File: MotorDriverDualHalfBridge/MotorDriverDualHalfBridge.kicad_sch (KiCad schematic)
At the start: 42 parts, among them J3 Batt+, J3 Batt-, J3 Motor Bottom Connection, J3 Motor Middle Connection, J3 Motor Upper Connection, J6 Conn_01x04, Q1 IAUA250N04S6N005, Q2 IAUA250N04S6N005, U1 2ED21824S06J, U2 EL817, U3 EL817

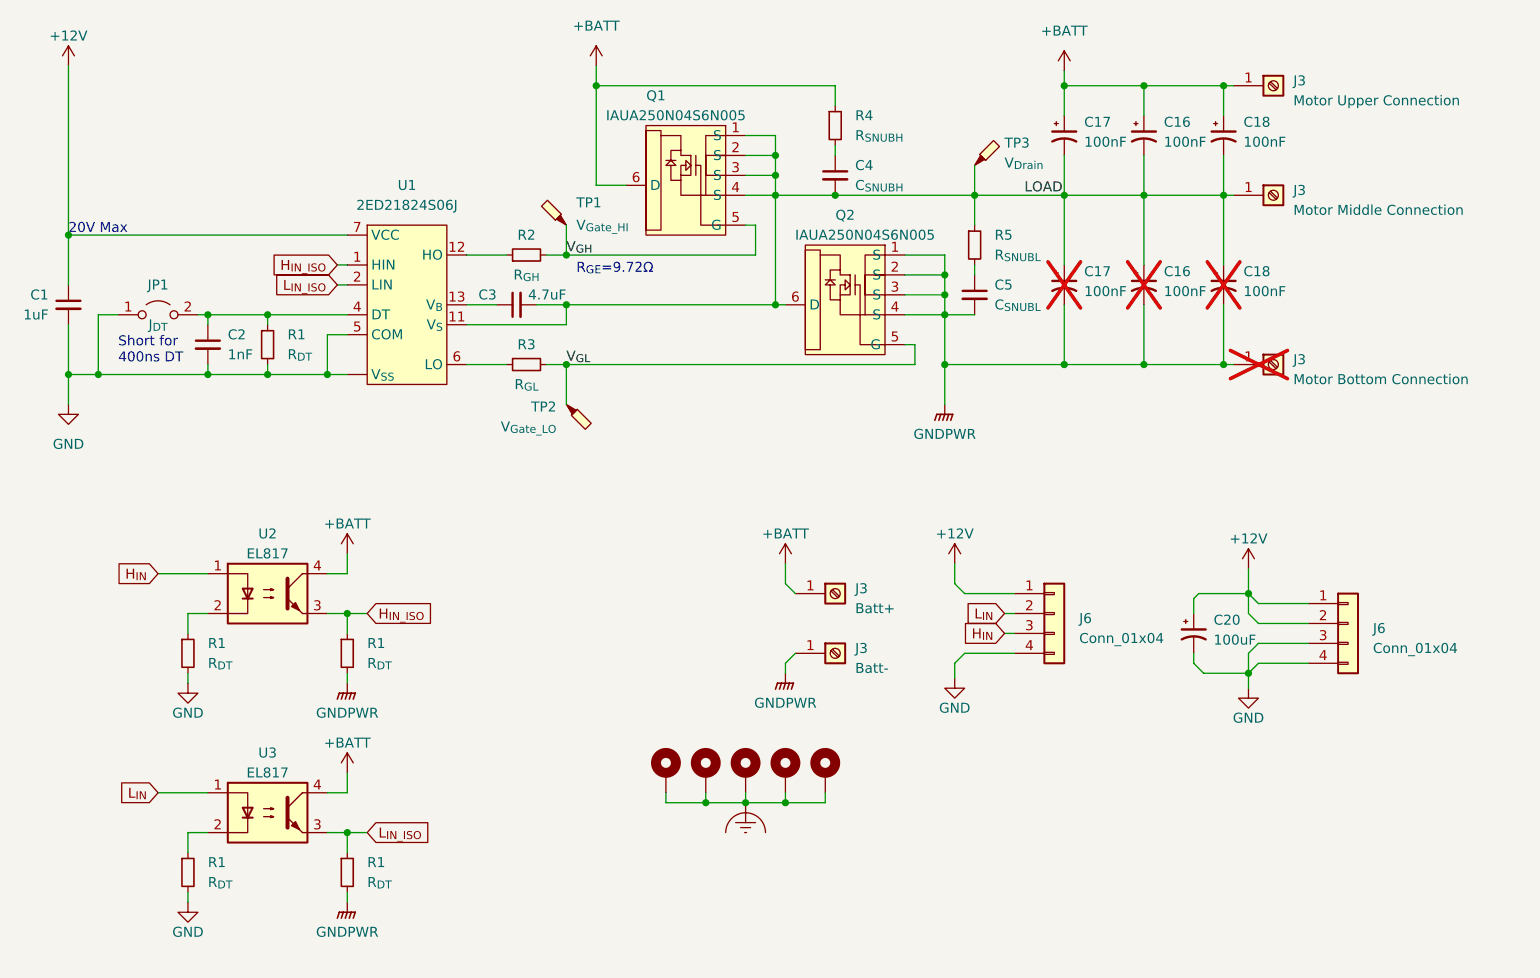
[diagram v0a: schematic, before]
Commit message: Motor Driver V1.01
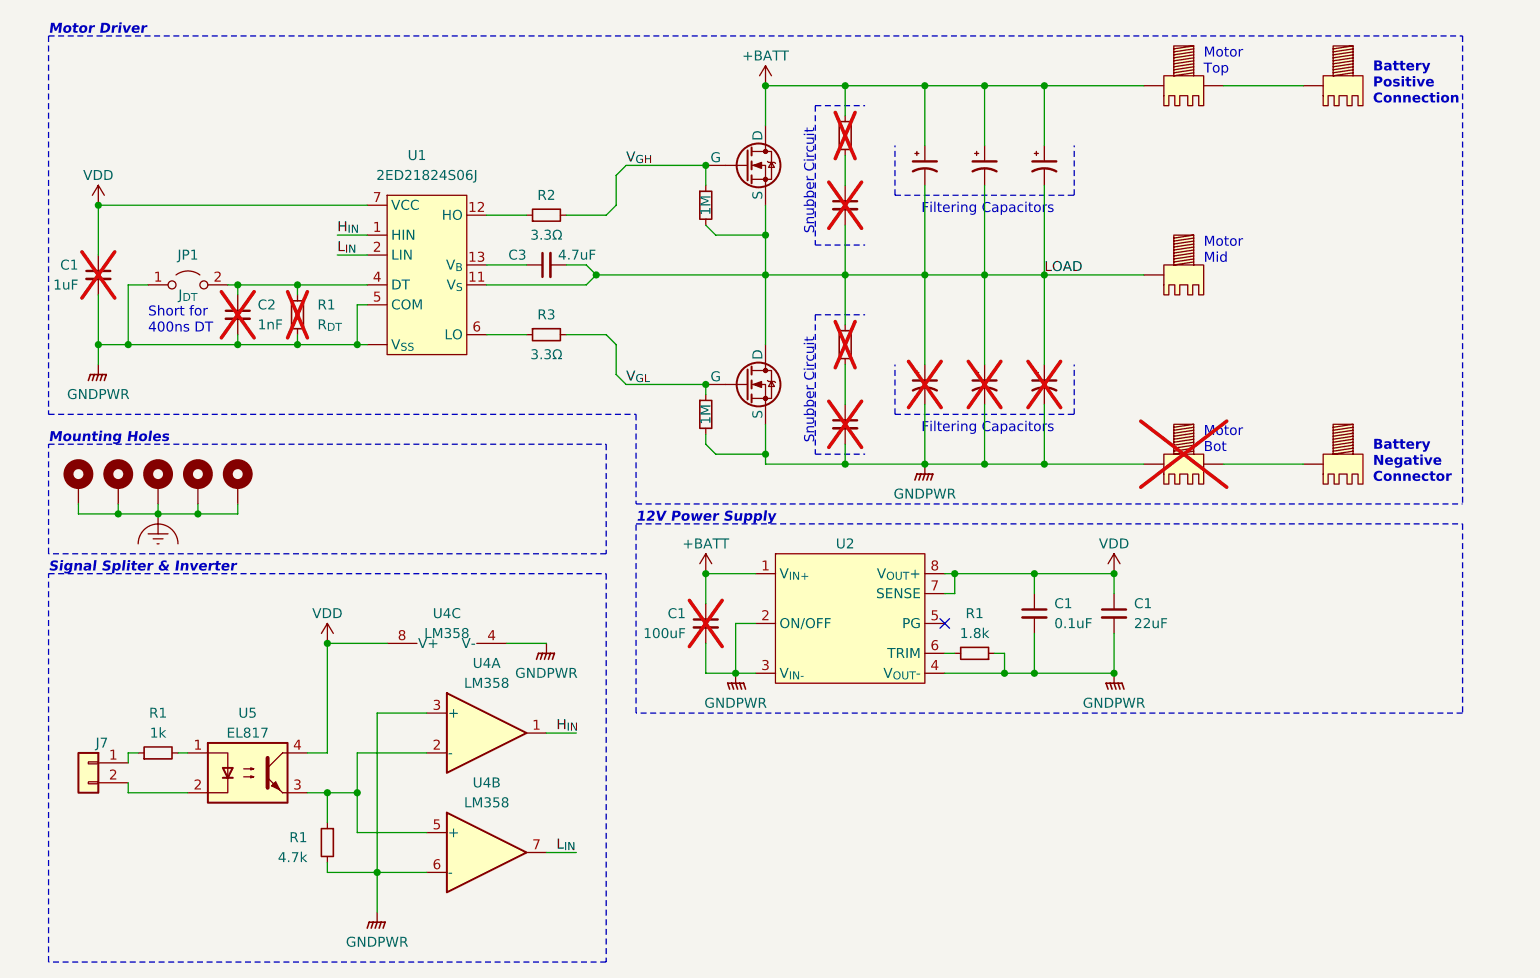
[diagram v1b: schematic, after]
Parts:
- removed C20: 100uF, Capacitor_SMD:CP_Elec_6.3x5.4_Nichicon, symbol Device:C_Polarized_Small_US
- removed J3: Motor Bottom Connection, Library:M5 Screw Terminal, symbol Connector:Screw_Terminal_01x01
- removed J3: Motor Upper Connection, Library:M5 Screw Terminal, symbol Connector:Screw_Terminal_01x01
- removed J3: Batt-, Library:M5 Screw Terminal, symbol Connector:Screw_Terminal_01x01
- removed J3: Motor Middle Connection, Library:M5 Screw Terminal, symbol Connector:Screw_Terminal_01x01
- removed J3: Batt+, Library:M5 Screw Terminal, symbol Connector:Screw_Terminal_01x01
- removed J6 (x2): Conn_01x04, Library:MOLEX_2078430004_L1NK_250_4-PIN, symbol Connector_Generic:Conn_01x04
- removed Q1, Q2: IAUA250N04S6N005, Library:IAUA250N04S6N005AUMA1, symbol MySymbols:IAUA250N04S6N005
- removed R1 (x4): R_{DT}, Resistor_THT:R_Axial_DIN0207_L6.3mm_D2.5mm_P10.16mm_Horizontal, symbol Device:R_Small
- removed TP1: V_{Gate_HI}, TestPoint:TestPoint_Pad_D1.0mm, symbol Connector:TestPoint_Probe
- removed TP2: V_{Gate_LO}, TestPoint:TestPoint_Pad_D1.0mm, symbol Connector:TestPoint_Probe
- removed TP3: V_{Drain}, TestPoint:TestPoint_Pad_D1.0mm, symbol Connector:TestPoint_Probe
- removed U2, U3: EL817, Package_DIP:DIP-4_W7.62mm, symbol Isolator:EL817
- added C1: 0.1uF, Capacitor_SMD:C_0603_1608Metric_Pad1.08x0.95mm_HandSolder, symbol Device:C_Small
- added C1: 100uF, Capacitor_SMD:C_Elec_5x5.8, symbol Device:C_Small
- added C1: 22uF, Capacitor_SMD:CP_Elec_5x5.8, symbol Device:C_Small
- added J1, J4, J5: ~, symbol My Global Library:M5_Screw_Terminal_Side
- added J2, J3: ~, symbol My Global Library:M5 Screw Terminal Both
- added J7: Conn_01x02, Connector_JST:JST_EH_B2B-EH-A_1x02_P2.50mm_Vertical, symbol Connector_Generic:Conn_01x02
- added Q1, Q2: NMOS, symbol Simulation_SPICE:NMOS
- added R1: 1k, Resistor_THT:R_Axial_DIN0207_L6.3mm_D2.5mm_P10.16mm_Horizontal, symbol Device:R_Small
- added R1: 4.7k, Resistor_THT:R_Axial_DIN0207_L6.3mm_D2.5mm_P10.16mm_Horizontal, symbol Device:R_Small
- added R1: 1.8k, Resistor_THT:R_Axial_DIN0207_L6.3mm_D2.5mm_P10.16mm_Horizontal, symbol Device:R_Small
- added R2 (x2): 1Μ, Resistor_SMD:R_0805_2012Metric_Pad1.20x1.40mm_HandSolder, symbol Device:R_Small
- added U2: ~, Library:I3A4W005A150V001R, symbol SymbolLibrary:U?
- added U4: LM358, Package_DIP:DIP-8_W7.62mm_LongPads, symbol Amplifier_Operational:LM358
- added U5: EL817, Package_DIP:DIP-4_W7.62mm, symbol Isolator:EL817
- C1, C2, C4, C5, R1, R4, R5: now not fitted
- R2: value R_{G}_{H} -> 3.3Ω
- R3: value R_{G}_{L} -> 3.3Ω
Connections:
- net GND is gone; now on net GNDPWR: C1.2, C2.2, JP1.1 (A), R1.2, U1. (V_{SS}), U1.5 (COM)
- net H_{IN}_{_ISO} is gone; now on net H_{IN}: U1.1 (HIN)
- net L_{IN}_{_ISO} is gone; now on net L_{IN}: U1.2 (LIN)
- net +BATT: now also C1.1, J3.1 (0), Q1.1 (D), U2.1 (V_{IN+})
- net GNDPWR: now also C1.2, C1.2, C1.2, J2.1 (0), Q2.3 (S), R1.1, R1.2, R2.2, U2.2 (ON/OFF), U2.3 (V_{IN-}), U2.4 (V_{OUT}-), U4.3 (+), U4.4 (V-), U4.6 (-)
- net H_{IN}: now also U4.1
- net LOAD: now also J1.1 (0), Q1.3 (S), Q2.1 (D), R2.2
- net L_{IN}: now also U4.7
- net V_{GH}: now also Q1.2 (G), R2.1
- net V_{GL}: now also Q2.2 (G), R2.1
- net +12V renamed VDD
- net VDD: now also C1.1, C1.1, U2.7 (SENSE), U2.8 (V_{OUT}+), U4.8 (V+), U5.4
- new net: R1.1, U4.2 (-), U4.5 (+), U5.3
- new net: J7.1 (Pin_1), R1.1
- new net: J7.2 (Pin_2), U5.2
- new net: R1.2, U5.1
- new net: J2.1 (0), J5.1 (0)
- new net: J3.1 (0), J4.1 (0)
- new net: R1.2, U2.6 (TRIM)
- no-connect marks 0 -> 1
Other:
- note added: "12V Power Supply"
- note added: "Battery Negative Connector"
- note added: "Battery Positive Connection"
- note added: "Filtering Capacitors"
- note added: "Motor Bot"
- note added: "Motor Driver"
- note added: "Motor Mid"
- note added: "Motor Top"
- note added: "Mounting Holes"
- note added: "Signal Spliter & Inverter"
- note added: "Snubber Circuit"
- note removed: "20V Max"
- note removed: "R_{GE}=9.72Ω"
- moved on the sheet: C3, JP1, R2, R3, U1
